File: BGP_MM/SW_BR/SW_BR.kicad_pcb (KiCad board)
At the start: 2 copper layers, 12 x 13 mm, 2 parts, among them P1 CONN_01X03, P2 CONN_01X02

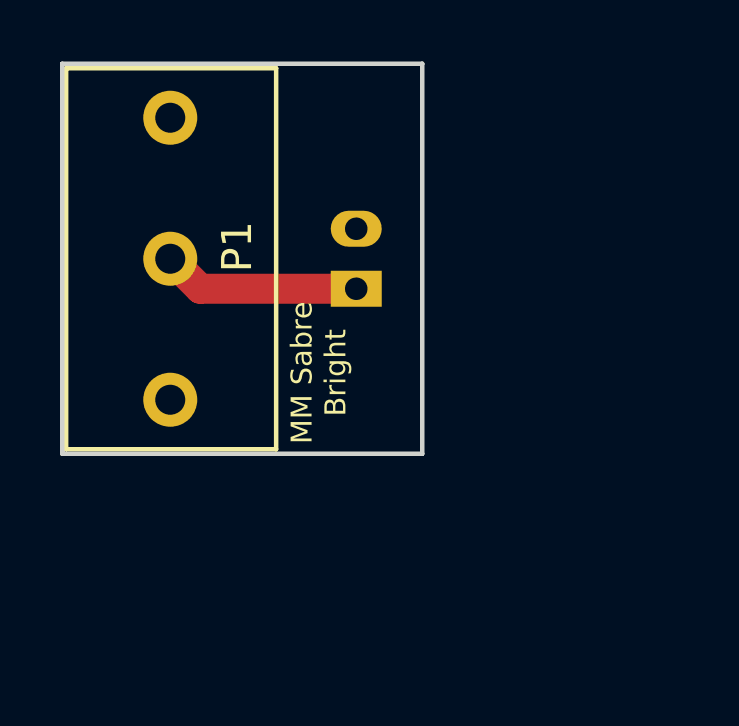
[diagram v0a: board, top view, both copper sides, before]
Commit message: MM Refactoring
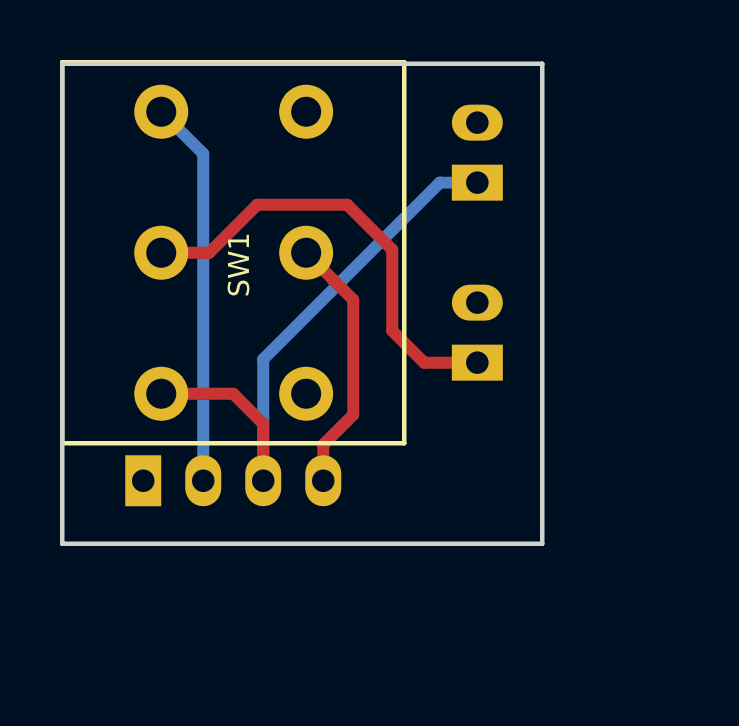
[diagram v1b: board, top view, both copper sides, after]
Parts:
- added P3: CONN_01X02, Connectors_JST:JST_PH_B2B-PH-K_02x2.00mm_Straight, B.Cu at (151.8, 110.0)
- added SW1: SW_DPDT, LIBS:NKK_DPDT, F.Cu at (146.1, 101.6)
- P1: value CONN_01X03 -> CONN_01X04; footprint LIBS:NKK_SPDT -> Connectors_JST:JST_PH_B4B-PH-K_04x2.00mm_Straight; moved to B.Cu
- moved P2 5.37 mm to (151.8, 104.0)
- moved P1 2.86 mm to (140.7, 113.9), turned to 0 degrees
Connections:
- P1 pad 2: Net-(P1-Pad2) -> /ACT_I
- P1 pad 3: Earth -> /SEL_I
- P2 pad 1: Net-(P1-Pad2) -> /SEL_I
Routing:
- net /SEL_I: track 0.00 -> 19.3 mm
- net /VOL_O: track 0.00 -> 15.0 mm
- net /ACT_I: track 0.00 -> 12.9 mm
- net /BR_I: track 0.00 -> 8.66 mm
- net Net-(P1-Pad2): track 6.61 -> 0.00 mm
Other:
- board size 12 x 13 mm -> 16 x 16 mm
- net class Default: clearance 0.2 -> 0.3; trace_width 0.25 -> 0.4
- rule trace_clearance: 0.2 -> 0.3
- board text removed: "MM Sabre Bright"

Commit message: MM Refactoring
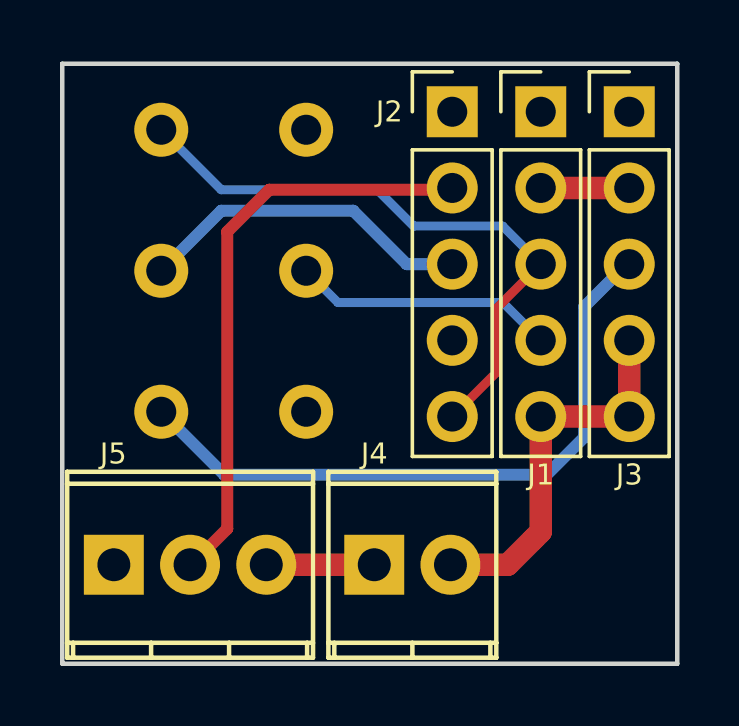
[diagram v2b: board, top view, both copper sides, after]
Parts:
- removed P1: CONN_01X04, Connectors_JST:JST_PH_B4B-PH-K_04x2.00mm_Straight
- removed P2, P3: CONN_01X02, Connectors_JST:JST_PH_B2B-PH-K_02x2.00mm_Straight
- added J1: Conn_01x05_Male, Pin_Headers:Pin_Header_Straight_1x05_Pitch2.54mm, F.Cu at (153.9, 101.6)
- added J2: Conn_01x05_Male, Pin_Headers:Pin_Header_Straight_1x05_Pitch2.54mm, F.Cu at (151.0, 101.6)
- added J3: Conn_01x05_Male, Pin_Headers:Pin_Header_Straight_1x05_Pitch2.54mm, F.Cu at (156.9, 101.6)
- added J4: Conn_01x02, LIBS:TerminalBlock_Phoenix_MPT-2.54mm_2pol, F.Cu at (148.4, 116.7)
- added J5: Conn_01x03, LIBS:TerminalBlock_Phoenix_MPT-2.54mm_3pol, F.Cu at (139.7, 116.7)
- SW1: moved to B.Cu
- moved SW1 10.0 mm to (146.1, 111.6), turned to 270 degrees
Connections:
- SW1 pad 1: Net-(SW1-Pad1) -> Earth
- SW1 pad 2: /BR_I -> /BR
- SW1 pad 3: Earth -> Net-(SW1-Pad3)
- SW1 pad 4: /ACT_I -> /MID
- SW1 pad 5: /VOL_O -> /VOL_I
- SW1 pad 6: /SEL_I -> /SEL
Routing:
- net /MID: track 0.00 -> 21.9 mm
- net /SEL: track 0.00 -> 20.8 mm
- net /SEL_I: track 19.3 -> 0.00 mm
- net /ACT_I: track 12.9 -> 0.00 mm
- net VCC: track 0.00 -> 12.8 mm
- net /VOL_I: track 0.00 -> 11.3 mm
- net /BR: track 0.00 -> 8.78 mm
- net /BR_I: track 8.66 -> 0.00 mm
- net /VOL_O: track 15.0 -> 19.7 mm
- net Net-(J4-Pad1): track 0.00 -> 3.60 mm
- net /ACT: track 0.00 -> 2.95 mm
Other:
- board size 16 x 16 mm -> 20.5 x 20 mm
- net class Default: clearance 0.3 -> 0.26; trace_width 0.4 -> 0.3
- rule trace_clearance: 0.3 -> 0.26
